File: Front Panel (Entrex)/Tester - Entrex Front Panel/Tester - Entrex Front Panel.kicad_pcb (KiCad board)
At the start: 2 copper layers, 114 x 99 mm, 15 parts, among them J1 Logic 8 CH, J10 Conn_02x26_Top_Bottom, J11 Logic 8 CH, J12 Logic 8 CH, J2 Conn_01x04, J3 Conn_01x08, J4 Conn_01x08, J5 Conn_01x06, J6 Conn_01x04, J7 Conn_01x02, J8 Conn_01x19, J9 Logic 8 CH, SW1 Reset

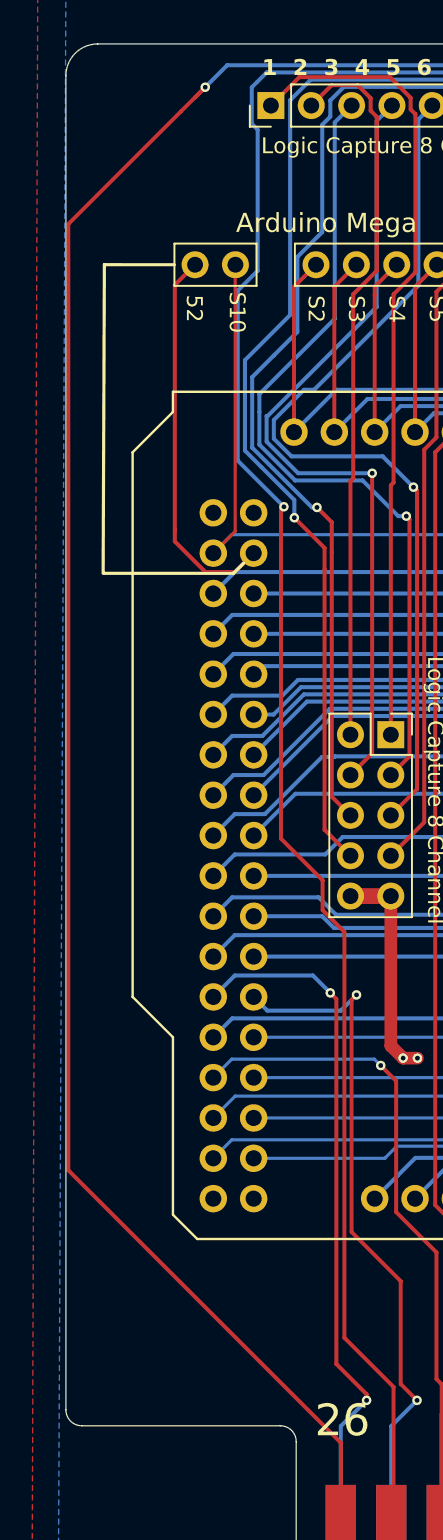
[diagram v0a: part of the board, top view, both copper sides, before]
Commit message: mmm
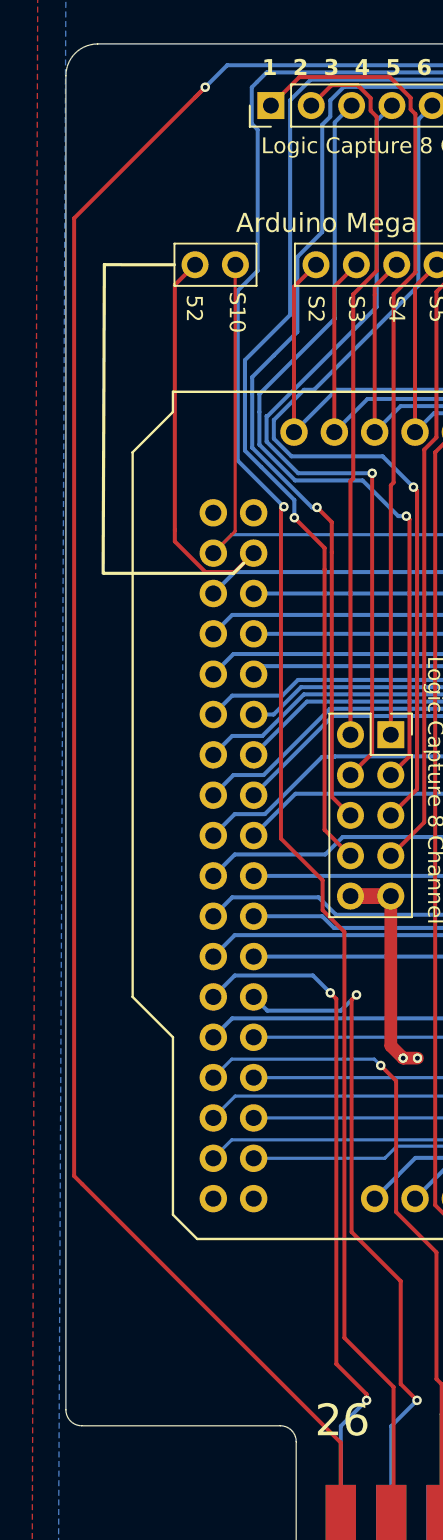
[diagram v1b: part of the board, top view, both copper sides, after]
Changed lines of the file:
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@@
     (solder_mask_min_width 0.25)
     (pcbplotparams
-      (layerselection 0x00010fc_ffffffff)
+      (layerselection 0x00310fc_ffffffff)
       (plot_on_all_layers_selection 0x0000000_00000000)
       (disableapertmacros false)
@@
   (segment (start 81.788 56.644) (end 83.176 55.256) (width 0.254) (layer "F.Cu") (net 45))
   (segment (start 52.705 44.704) (end 53.467 43.942) (width 0.25) (layer "F.Cu") (net 46))
-  (segment (start 44.718 52.691) (end 51.816 45.593) (width 0.25) (layer "F.Cu") (net 46))
+  (segment (start 45.085 112.623) (end 45.606 113.144) (width 0.25) (layer "F.Cu") (net 46))
   (segment (start 52.705 44.704) (end 53.34 44.069) (width 0.25) (layer "F.Cu") (net 46))
-  (segment (start 51.816 45.593) (end 52.705 44.704) (width 0.25) (layer "F.Cu") (net 46))
-  (segment (start 61.875 129.413) (end 44.718 112.256) (width 0.25) (layer "F.Cu") (net 46))
+  (segment (start 61.875 129.413) (end 45.606 113.144) (width 0.25) (layer "F.Cu") (net 46))
+  (segment (start 45.085 52.324) (end 45.085 112.623) (width 0.25) (layer "F.Cu") (net 46))
+  (segment (start 52.705 44.704) (end 45.085 52.324) (width 0.25) (layer "F.Cu") (net 46))
   (segment (start 61.875 136.22) (end 61.875 129.413) (width 0.25) (layer "F.Cu") (net 46))
-  (segment (start 44.718 112.256) (end 44.718 52.691) (width 0.25) (layer "F.Cu") (net 46))
   (via (at 53.34 44.069) (size 0.6) (drill 0.3) (layers "F.Cu" "B.Cu") (net 46))
   (segment (start 57.404 42.686) (end 54.723 42.686) (width 0.254) (layer "B.Cu") (net 46))
